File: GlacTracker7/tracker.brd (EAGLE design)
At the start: 120 x 89.3 mm, 84 parts, among them J1 THING_PLUS_PHYSICAL, Q1 2N3906, Q2 DMG6602SVT, Q3 DMG6602SVT, Q6 MMBT3906LT1SMD, Q7 DMG6602SVT, U2 FONA-800-BREAKOUT, U3 MP2155GQ-Z, U4 SPARKFUN-SWARM-M138, U5 SPARKFUN-GPS-ZED-F9P, U6 MP2155GQ-Z, U7 DS3231SN, U8 BQ24074QFN_3X3

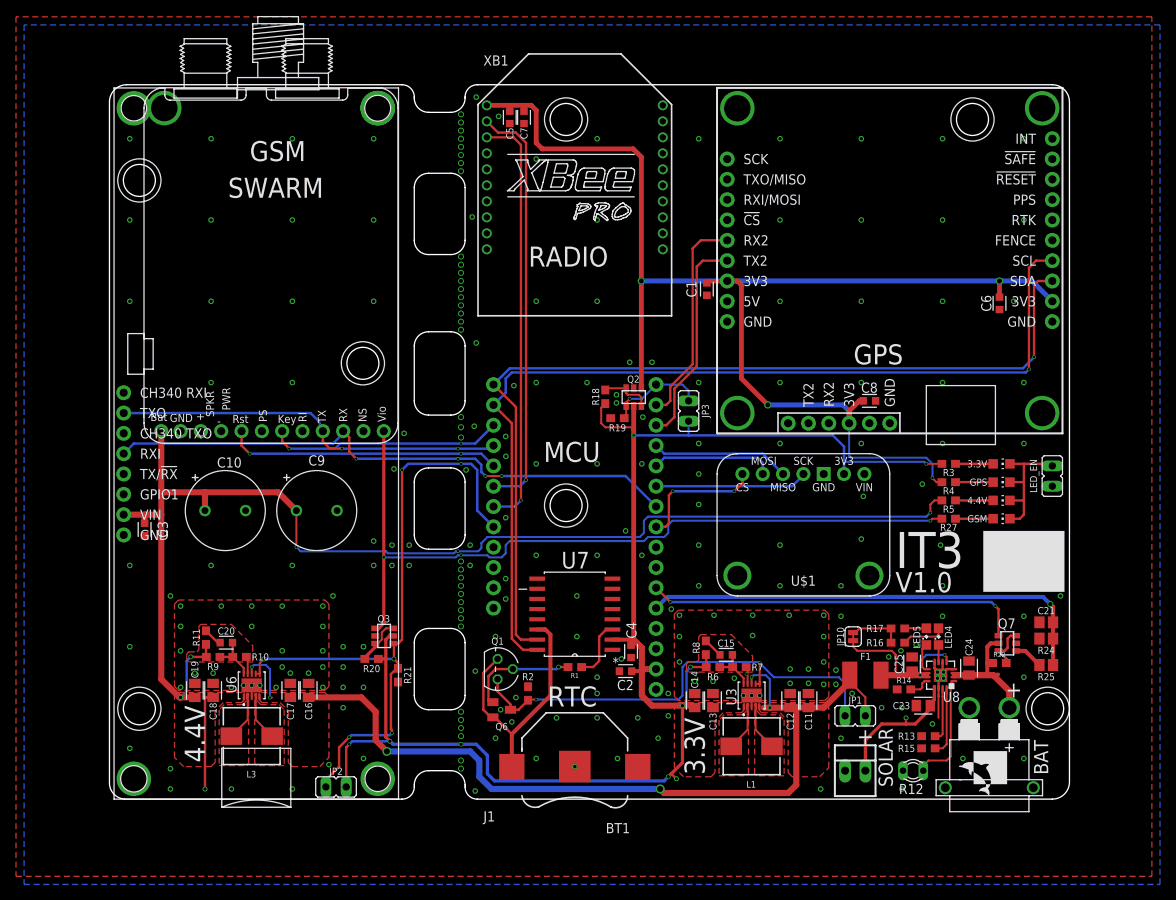
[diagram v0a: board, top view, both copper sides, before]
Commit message: missed and airwire
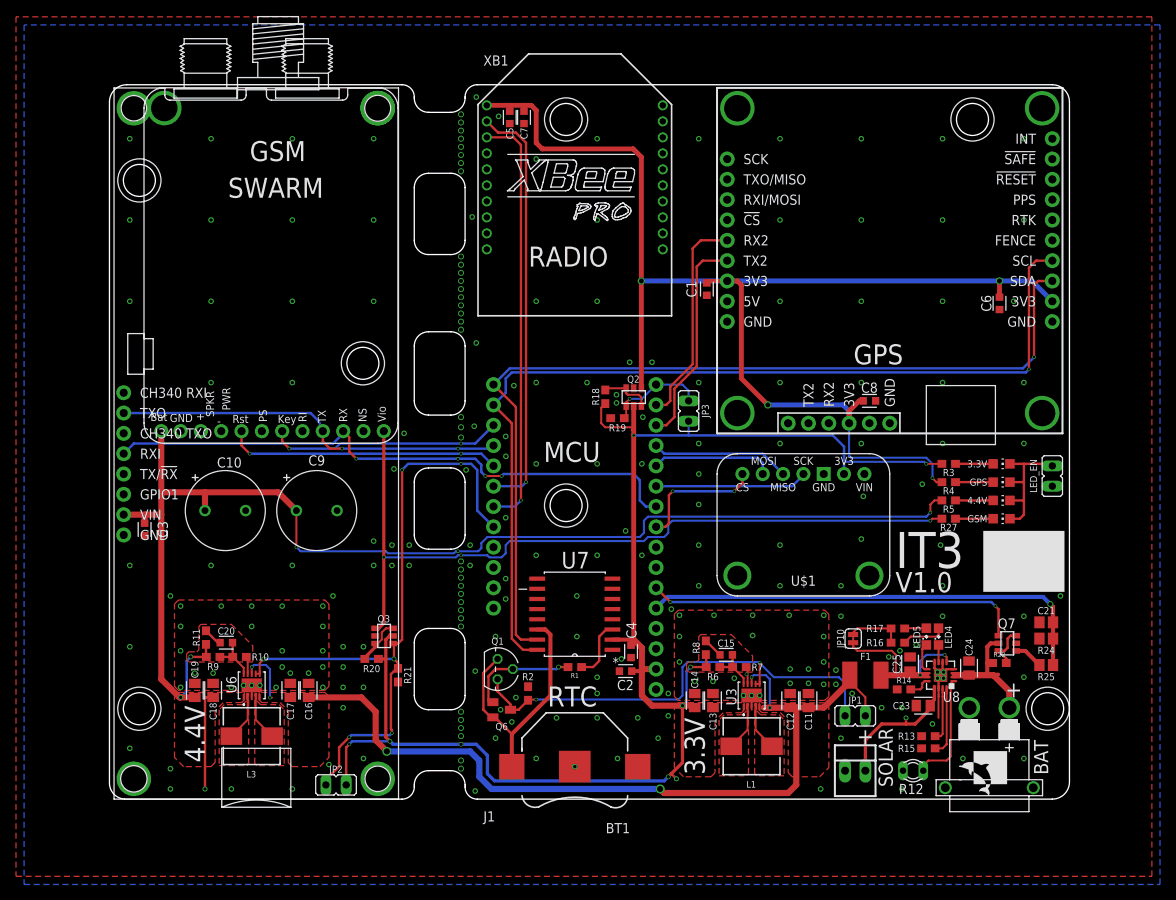
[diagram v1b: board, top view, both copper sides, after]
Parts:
- moved C25 0.25 mm to (100.1, 16.9)
- moved JP10 0.25 mm to (93.0, 20.1)
- moved JP2 0.25 mm to (28.3, 1.78)
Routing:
- net COMMS_RX: track 75.4 -> 77.1 mm
